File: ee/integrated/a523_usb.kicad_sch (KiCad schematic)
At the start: 5 parts, among them U201 A523

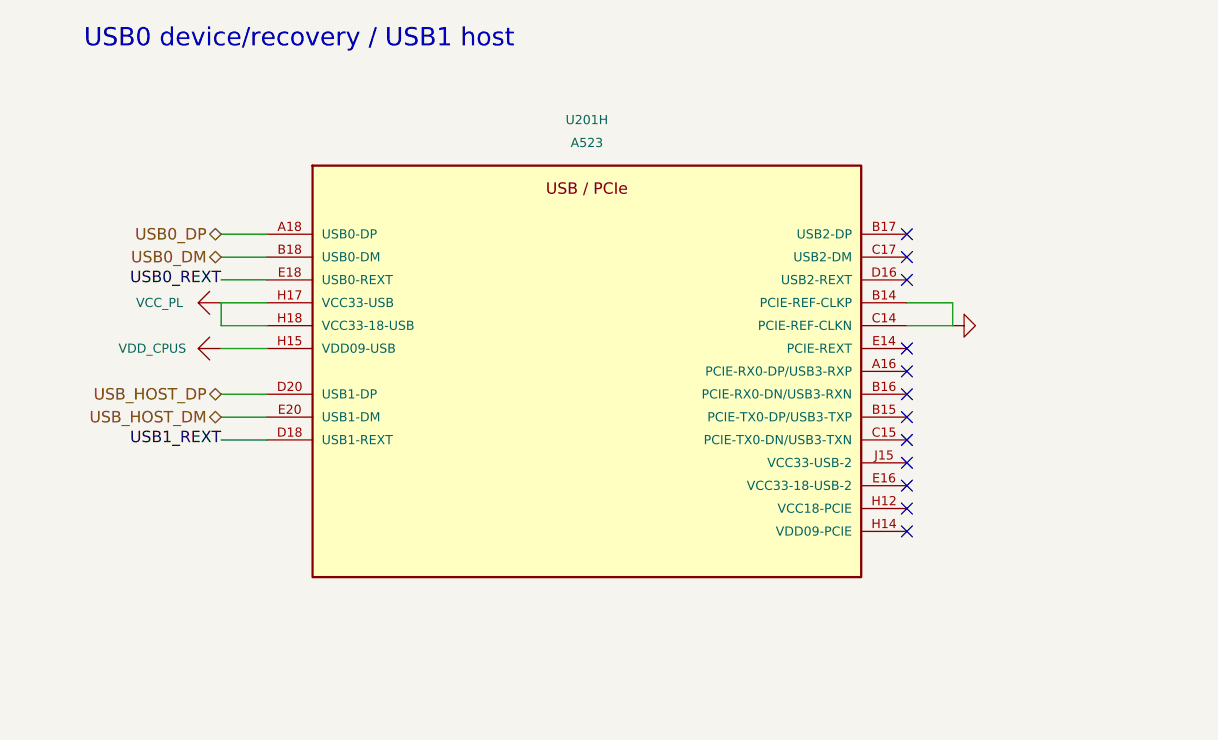
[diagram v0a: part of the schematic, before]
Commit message: Working on the schematic.
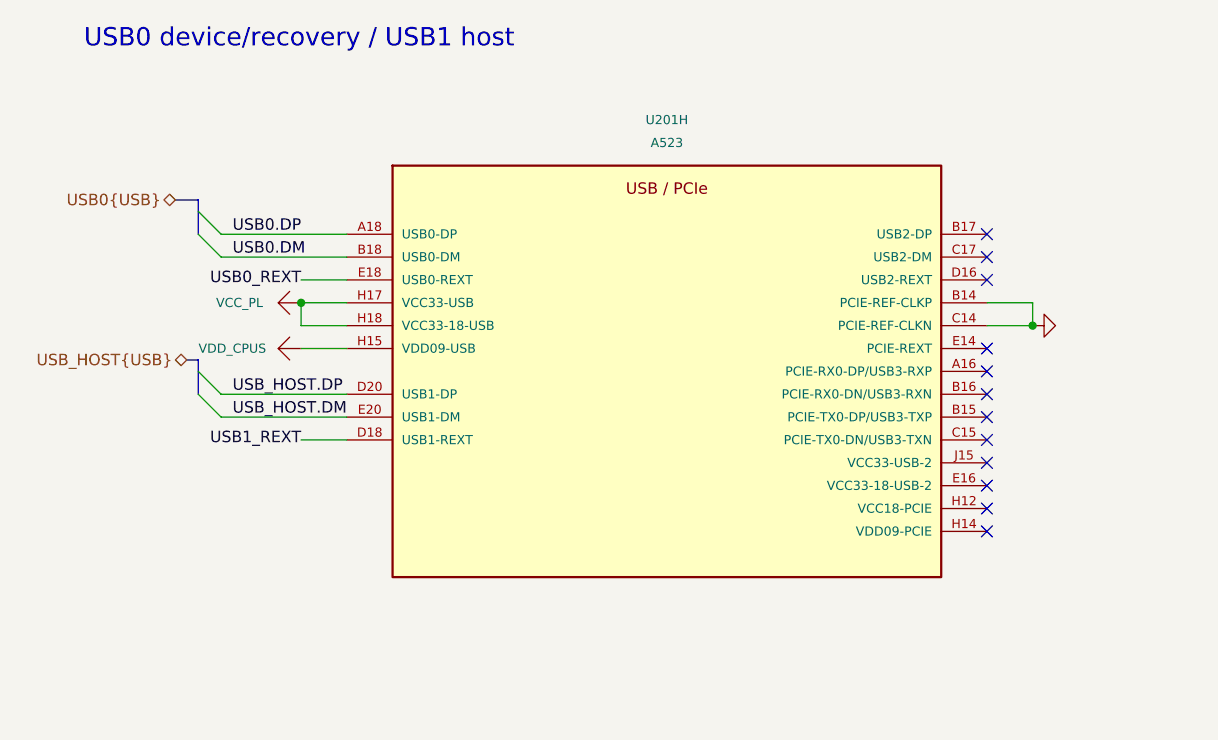
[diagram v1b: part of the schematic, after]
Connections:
- net USB0_DM renamed USB0.DM
- net USB0_DP renamed USB0.DP
- net USB_HOST_DM renamed USB_HOST.DM
- net USB_HOST_DP renamed USB_HOST.DP
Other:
- moved on the sheet: U201H
